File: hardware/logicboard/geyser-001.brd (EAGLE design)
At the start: 47 x 47 mm, 13 parts, among them T1 2SC1815

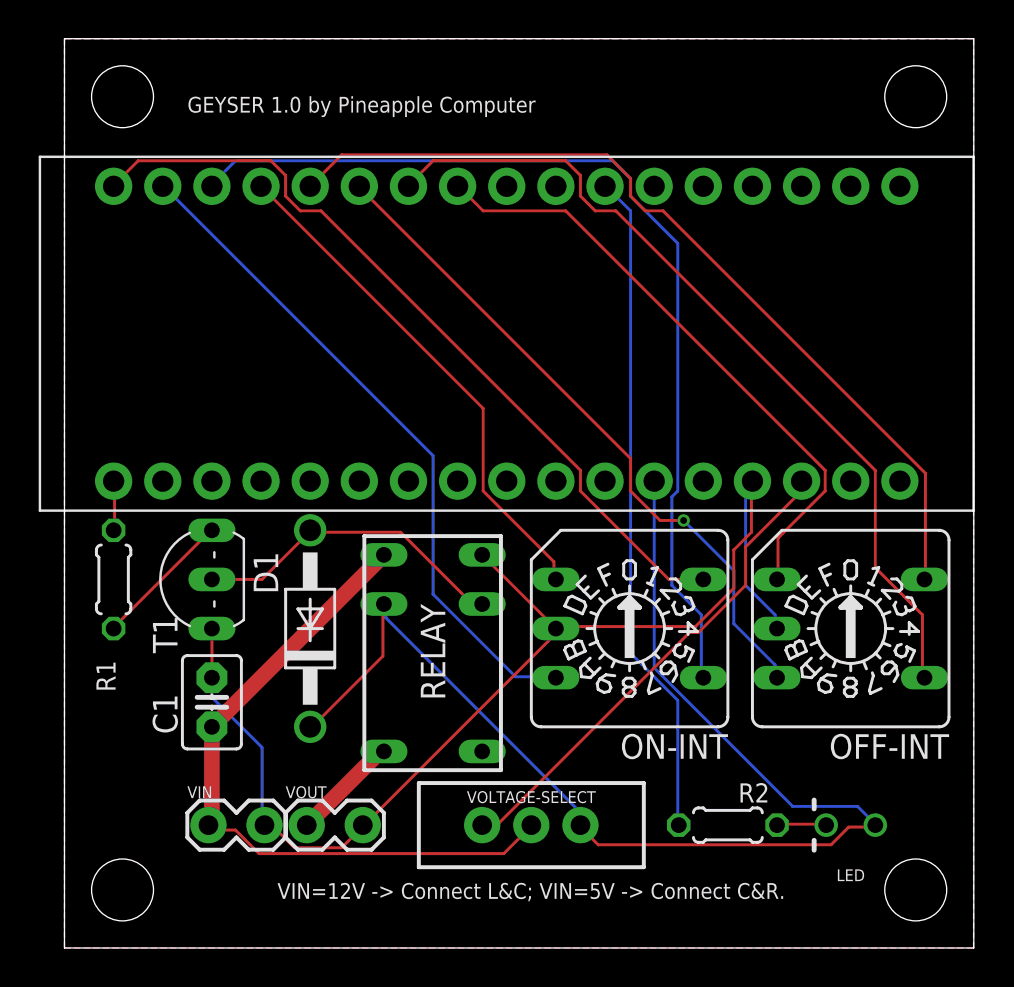
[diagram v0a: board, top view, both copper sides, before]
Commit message: Refined the board.
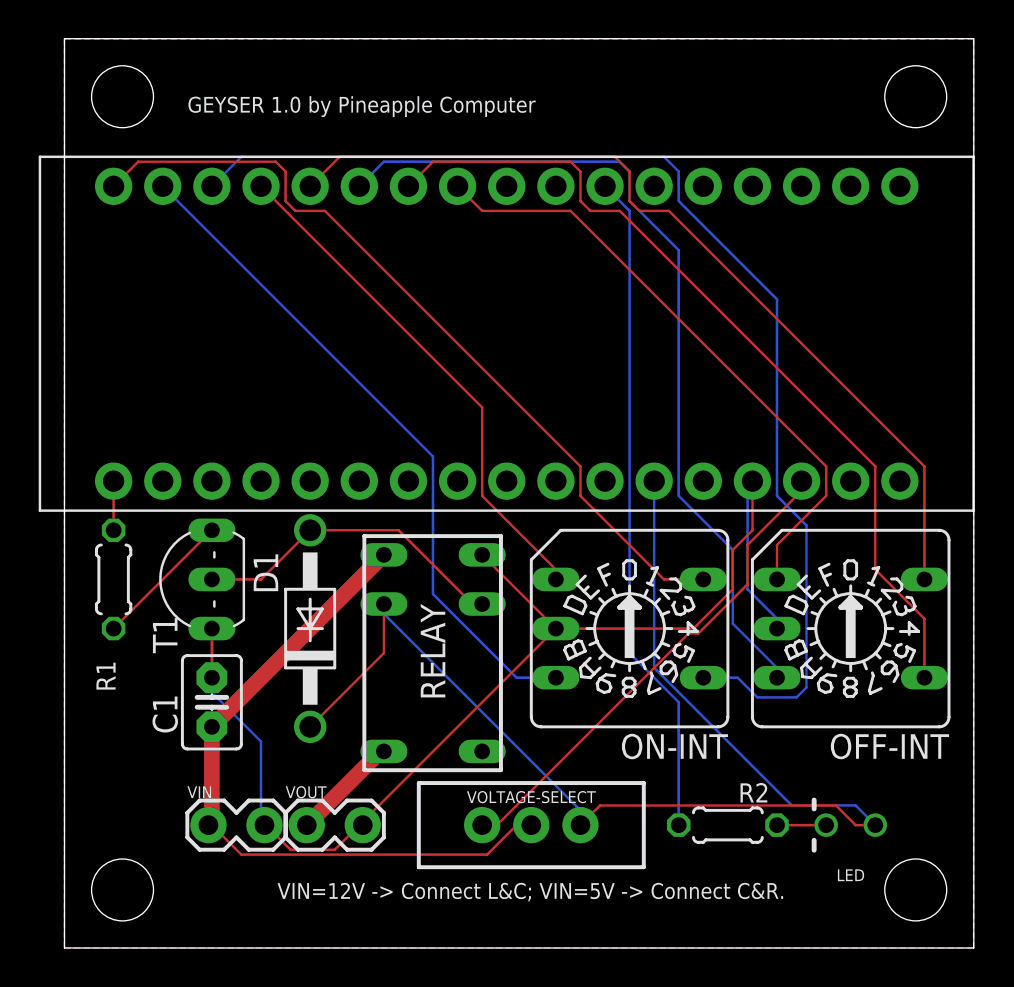
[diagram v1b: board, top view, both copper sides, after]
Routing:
- net N$9: track 50.3 -> 60.4 mm
- net N$5: track 35.1 -> 44.0 mm, vias 1 -> 0
